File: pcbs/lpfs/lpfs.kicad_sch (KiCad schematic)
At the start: 70 parts, among them K1 G6K-2F-Y, K10 G6K-2F-Y, K2 G6K-2F-Y, K3 G6K-2F-Y, K4 G6K-2F-Y, K5 G6K-2F-Y, K6 G6K-2F-Y, K7 G6K-2F-Y, K8 G6K-2F-Y, K9 G6K-2F-Y

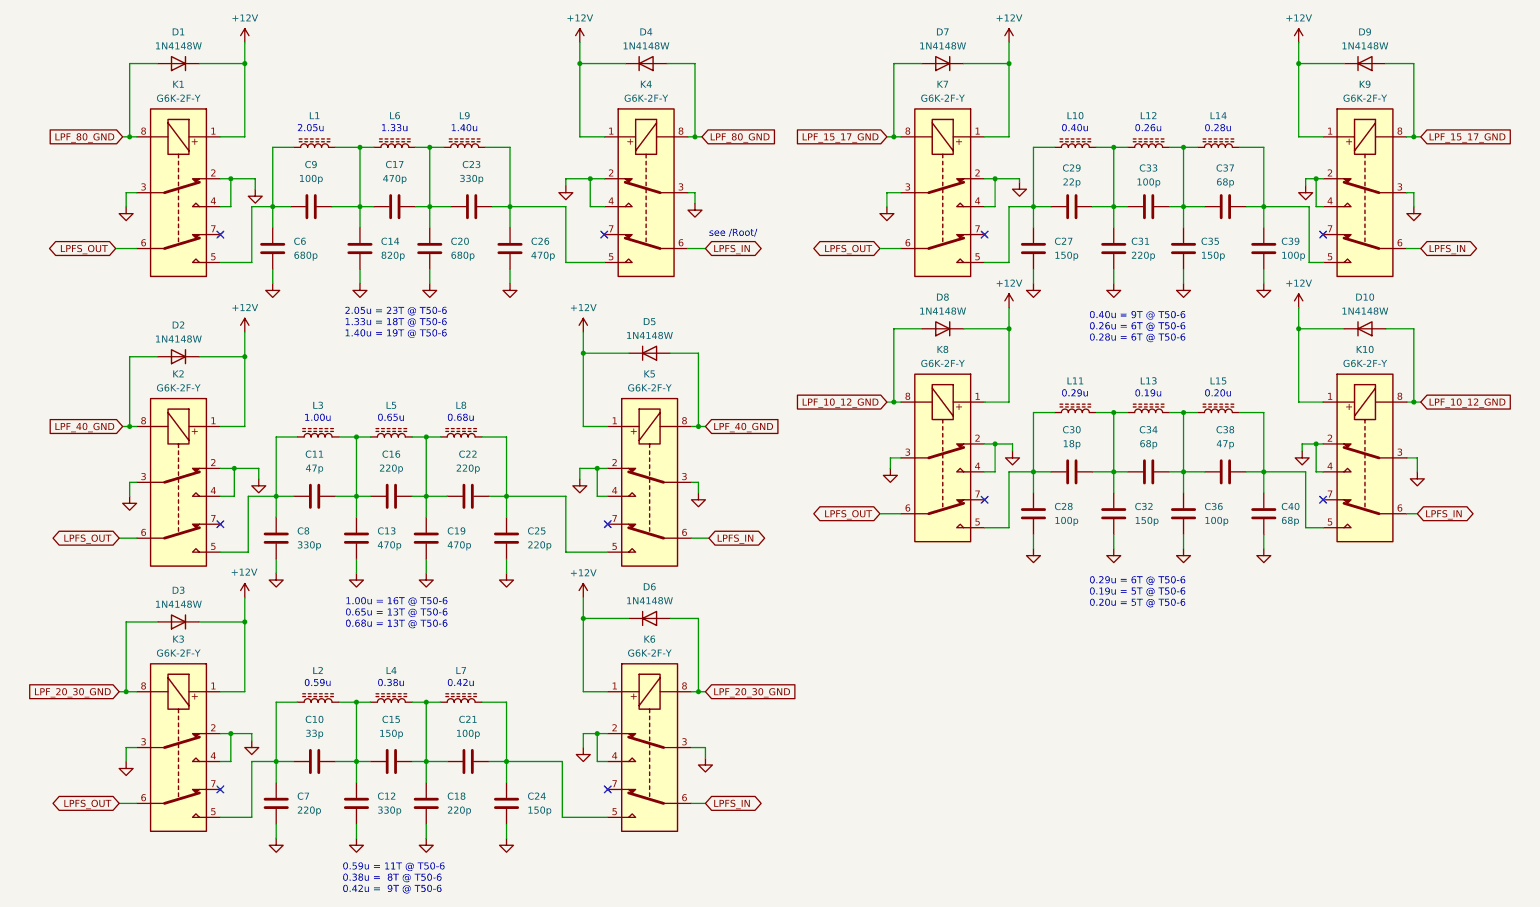
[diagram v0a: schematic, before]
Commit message: Minor changes
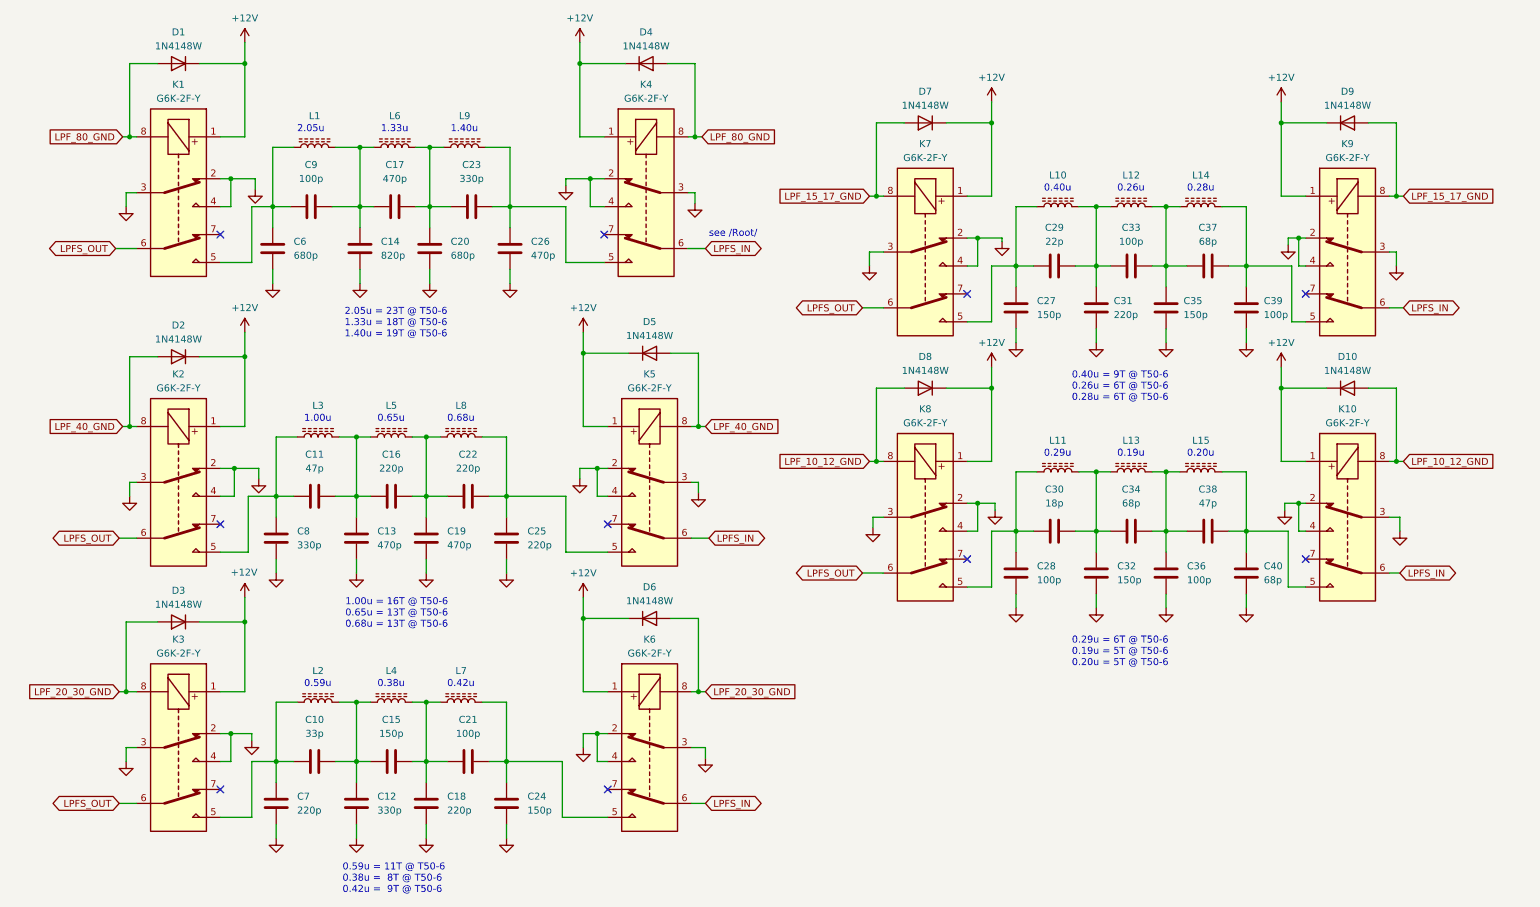
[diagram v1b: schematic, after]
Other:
- moved on the sheet: C27, C28, C29, C30, C31, C32, C33, C34, C35, C36, C37, C38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
